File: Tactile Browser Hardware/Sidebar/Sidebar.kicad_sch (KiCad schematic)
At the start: 22 parts, among them J1 Conn_01x02_Pin, J2 Conn_01x02_Pin, J3 Barrel_Jack_Switch, Q1 Q_PMOS_SGD, SW6 SW_Push, SW7 SW_Push, U2 74HC595

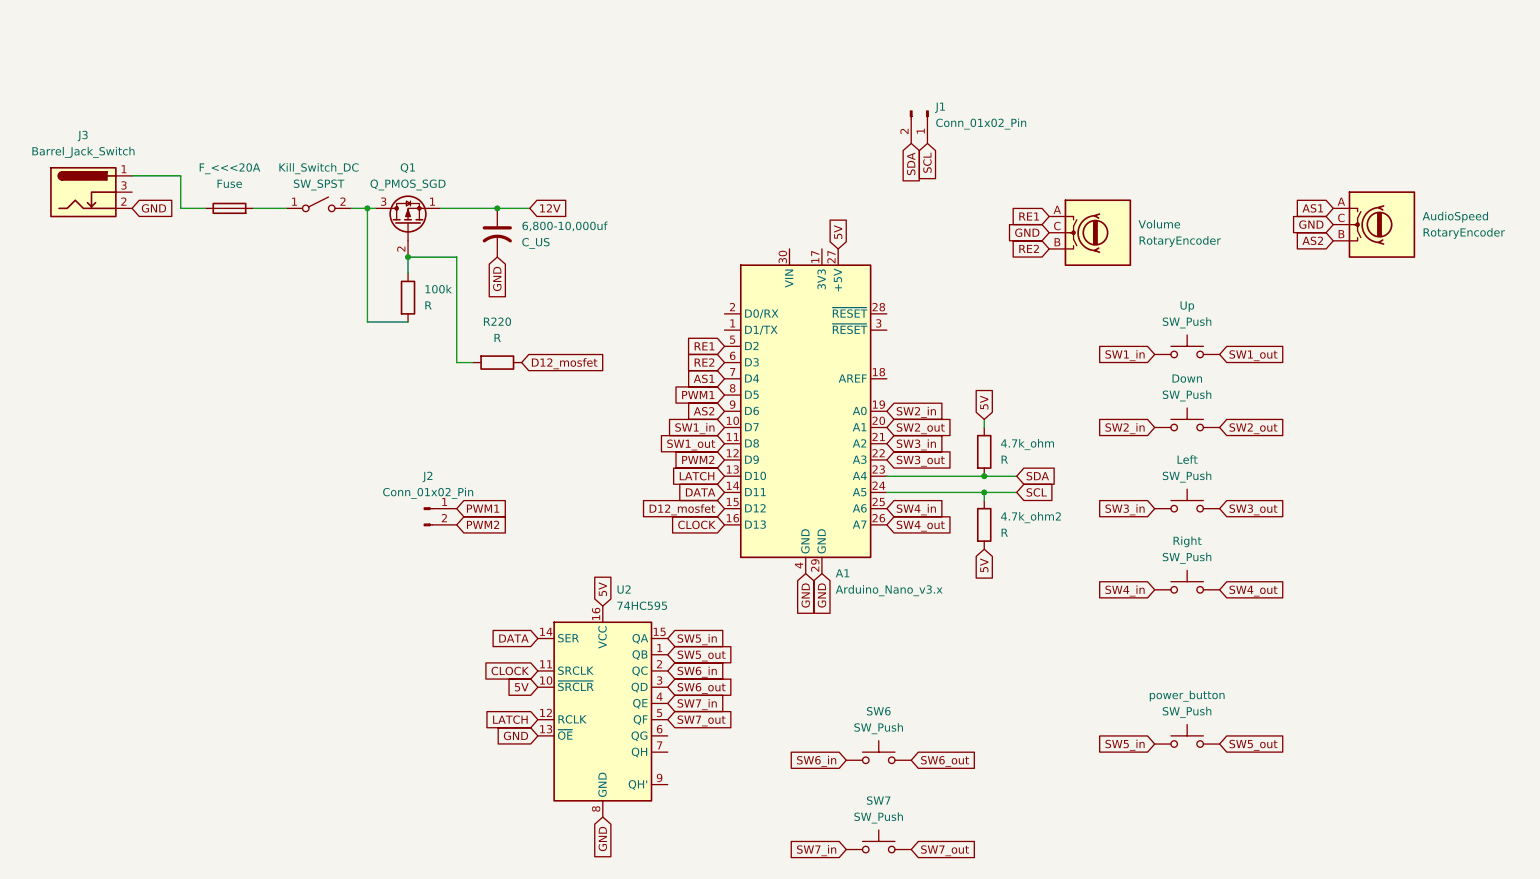
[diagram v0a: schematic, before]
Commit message: sidebar updates
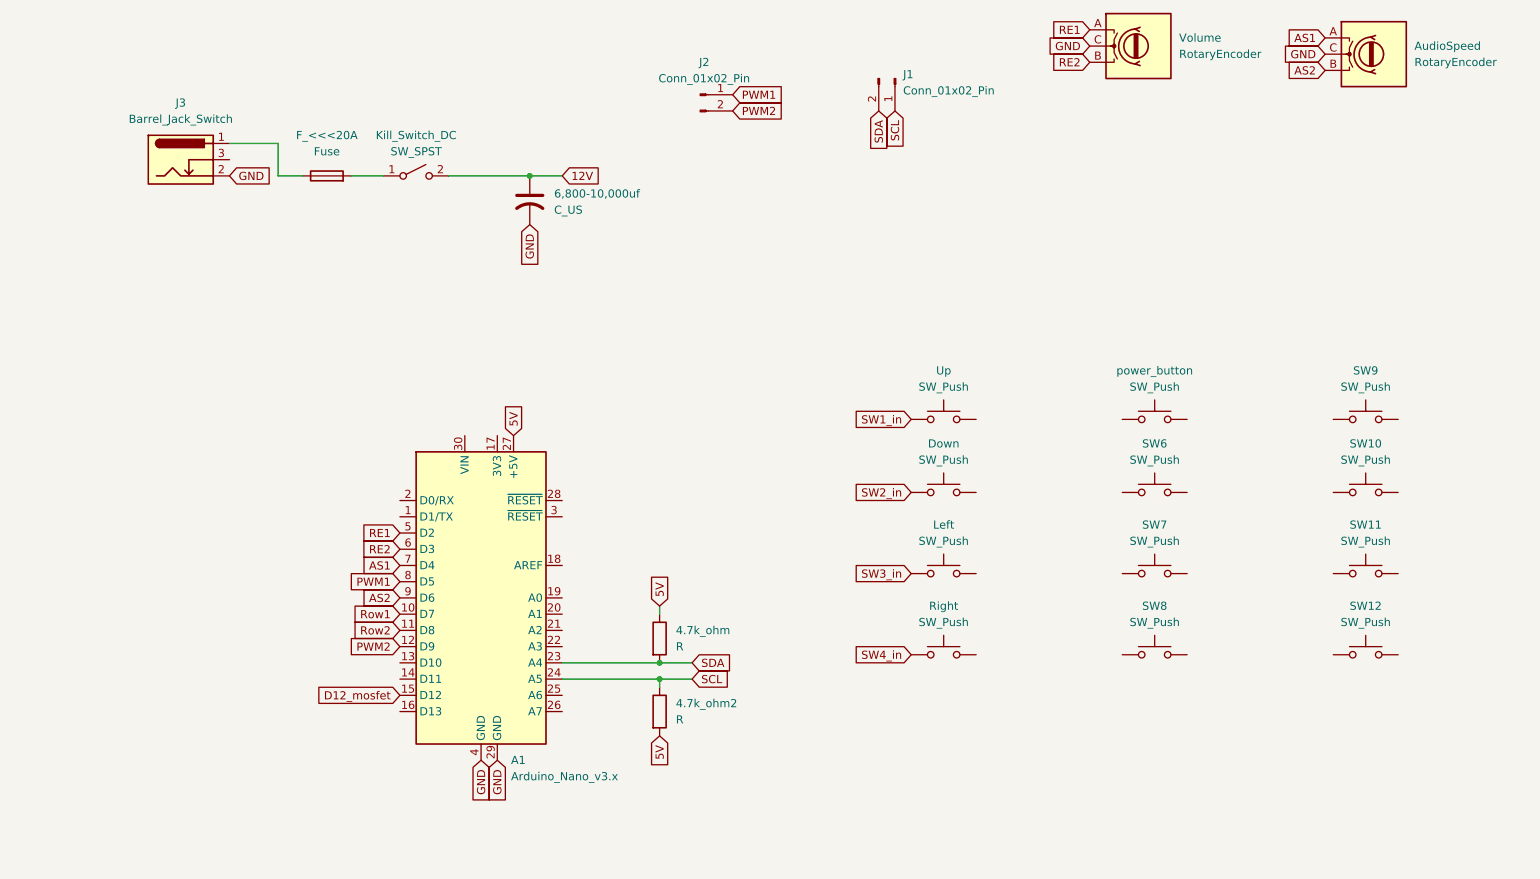
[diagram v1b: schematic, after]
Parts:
- removed 100k, R220: R, symbol Device:R
- removed Q1: Q_PMOS_SGD, symbol Transistor_FET:Q_PMOS_SGD
- removed U2: 74HC595, symbol 74xx:74HC595
- added SW10, SW11, SW12, SW8, SW9: SW_Push, symbol Switch:SW_Push
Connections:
- net 12V: now also Kill_Switch_DC.2 (B)
- net SW1_in: no longer A1.10 (D7)
- net SW2_in: no longer A1.19 (A0)
- net SW3_in: no longer A1.21 (A2)
- net SW4_in: no longer A1.25 (A6)
- net CLOCK: no longer names the net of A1.16 (D13)
- net DATA: no longer names the net of A1.14 (D11)
- net LATCH: no longer names the net of A1.13 (D10)
- net SW1_out: no longer names the net of Up.2
- net SW1_out: no longer A1.11 (D8)
- net SW2_out: no longer names the net of A1.20 (A1)
- net SW2_out: no longer Down.2
- net SW3_out: no longer names the net of Left.2
- net SW3_out: no longer A1.22 (A3)
- net SW4_out: no longer names the net of A1.26 (A7)
- net SW4_out: no longer Right.2
- net SW5_in: no longer names the net of power_button.1
- net SW5_out: no longer names the net of power_button.2
- net SW6_in: no longer names the net of SW6.1
- net SW6_out: no longer names the net of SW6.2
- net SW7_in: no longer names the net of SW7.1
- net SW7_out: no longer names the net of SW7.2
- new net Row1: A1.10 (D7)
- new net Row2: A1.11 (D8)
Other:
- moved on the sheet: 4.7k_ohm, 4.7k_ohm2, 6,800-10,000uf, A1, AudioSpeed, Down, F_<<<20A, J1, J2, J3, Kill_Switch_DC, Left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
